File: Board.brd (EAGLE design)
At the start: 110.5 x 61 mm, 26 parts, among them IC1 BUF634U, IC2 LM555D, Q1 35A/25V/8.5mΩ, Q2 35A/25V/8.5mΩ, Q3 35A/25V/8.5mΩ, X3 MSTBV4

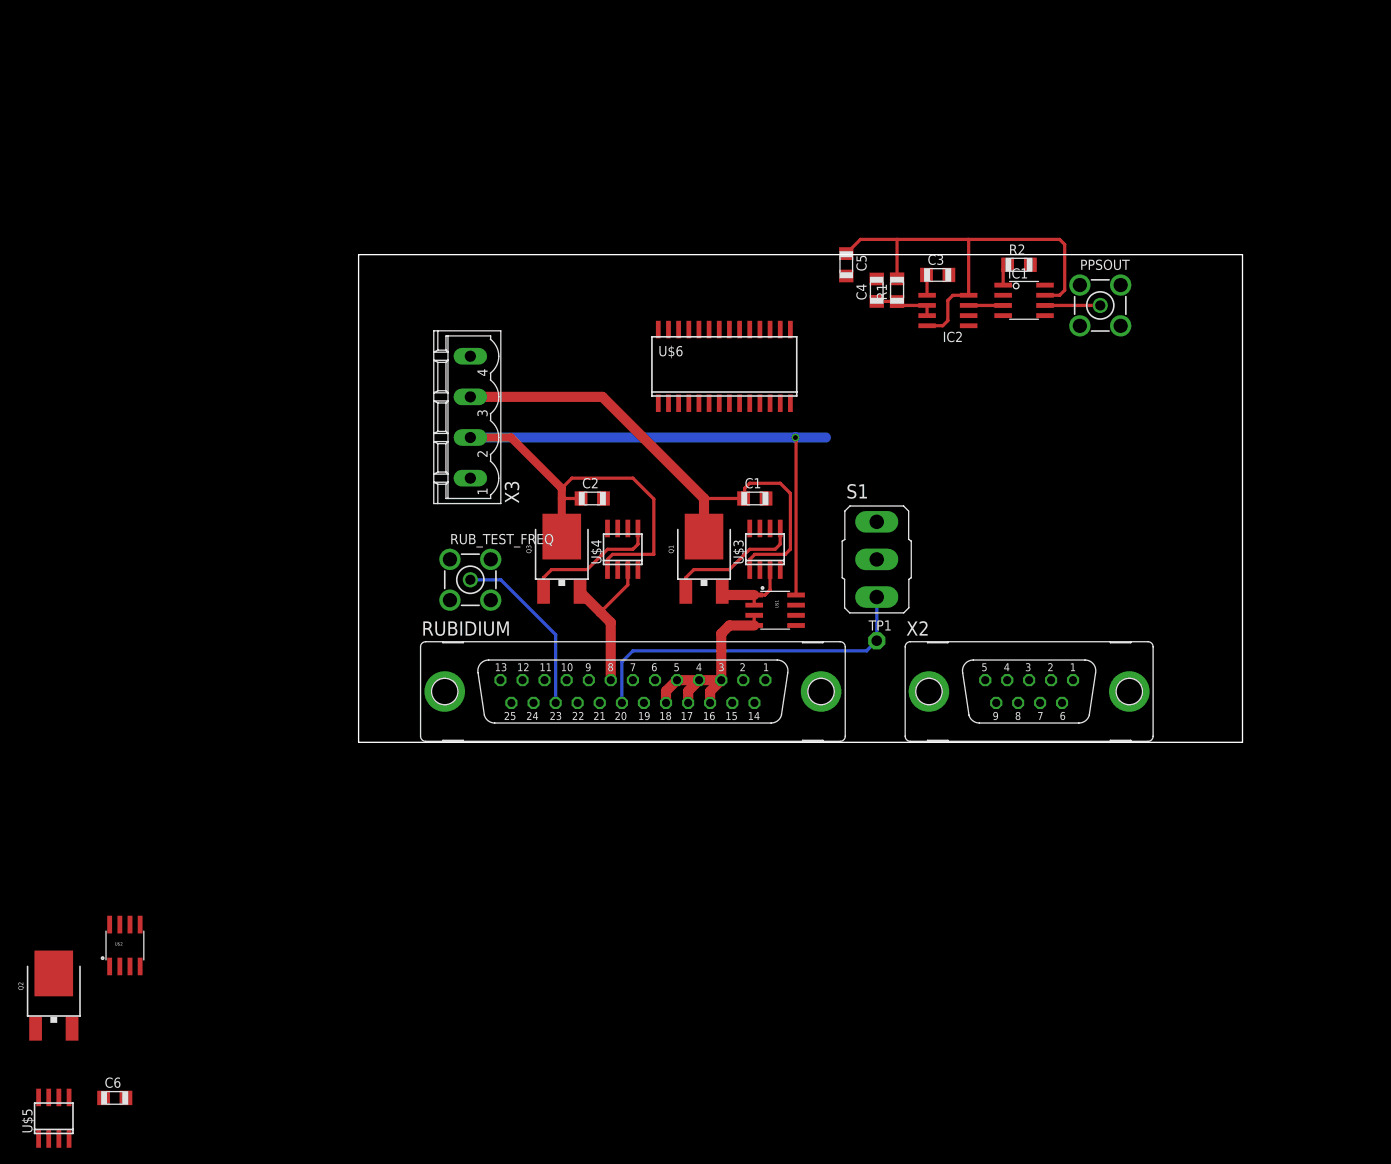
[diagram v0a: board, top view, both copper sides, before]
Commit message: PCB work
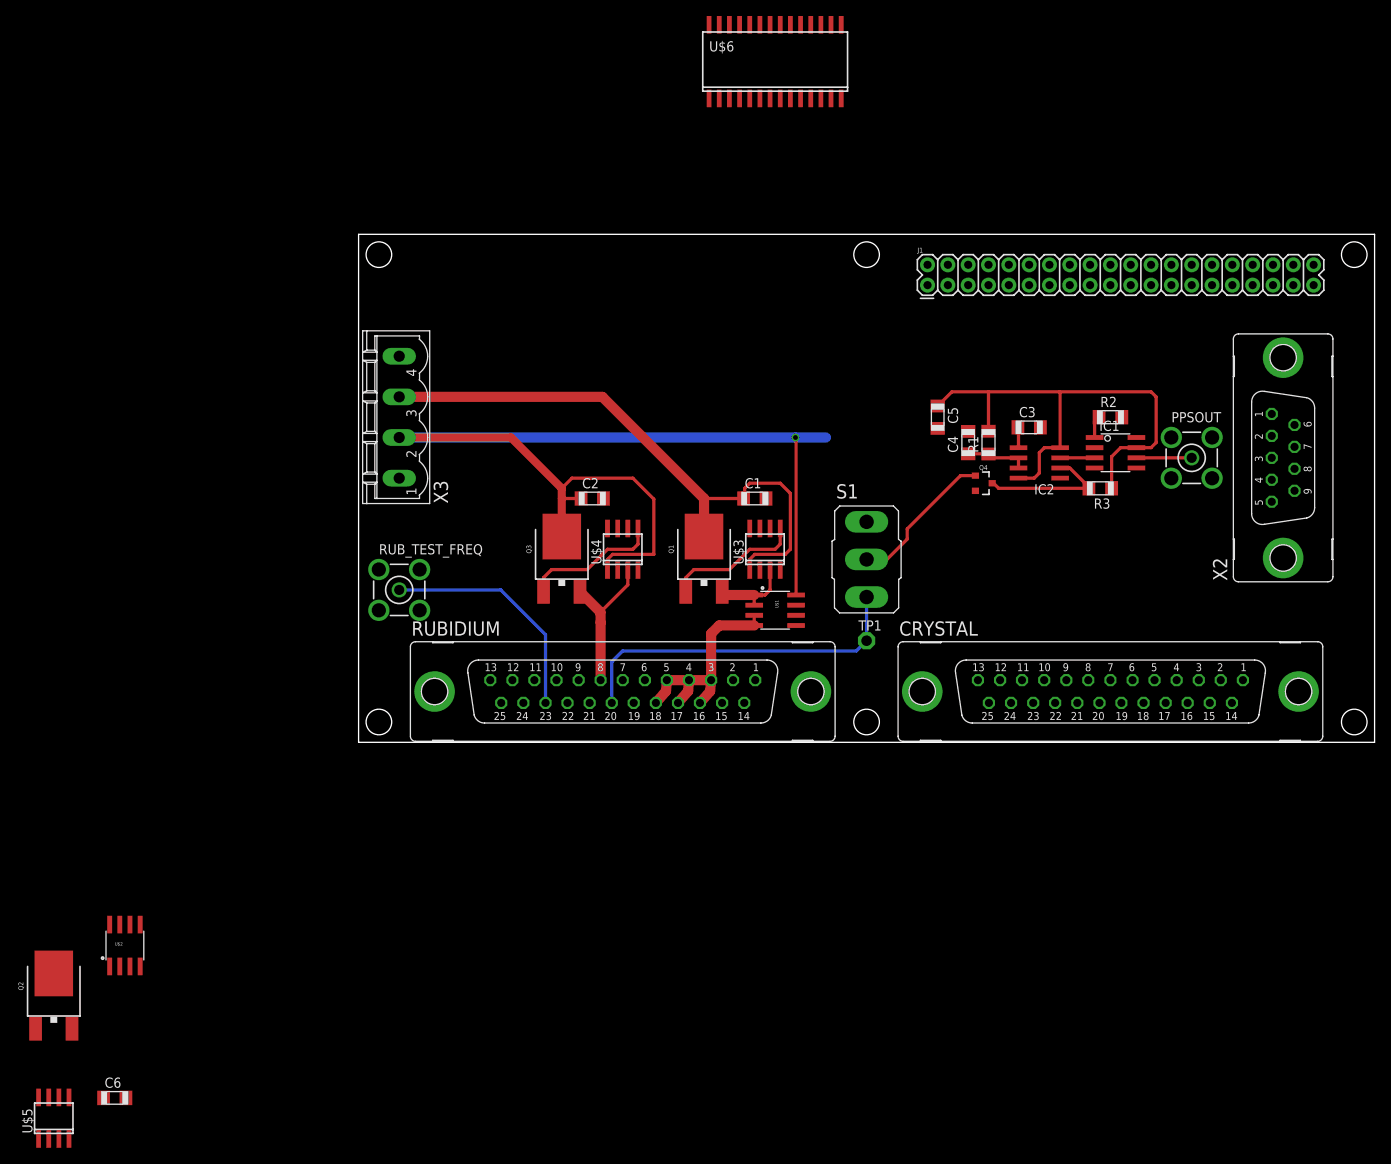
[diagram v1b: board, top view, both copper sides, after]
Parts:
- added CRYSTAL: (no value), con-subd:F25VP
- added J1: RASPBERRYPI-40-PIN-GPIO_PTH_NO_SHROUD, SparkFun-Connectors:2X20
- added Q4: 220mA/50V/3.5Ω, SparkFun-DiscreteSemi:SOT23-3
- added R3: 1k, resistor:R1206
- moved X2 43.1 mm to (115.6, 35.6), turned to 90 degrees
- moved U$6 38.6 mm to (52.1, 85.1)
- moved IC2 22.2 mm to (85.1, 34.9)
- moved C4 22.2 mm to (76.2, 37.5)
- moved PPSOUT 22.2 mm to (104.1, 35.6)
- moved R2 22.2 mm to (94.0, 40.6)
- moved C3 22.2 mm to (83.8, 39.4)
- moved C5 22.2 mm to (72.4, 40.6)
- moved IC1 22.2 mm to (94.6, 36.2)
- moved R1 22.2 mm to (78.7, 37.5)
- moved RUB_TEST_FREQ 8.98 mm to (5.08, 19.1)
- moved X3 8.89 mm to (5.08, 40.6)
- moved RUBIDIUM 1.27 mm to (33.0, 6.35)
- moved S1 1.27 mm to (63.5, 22.9)
- moved TP1 1.27 mm to (63.5, 12.7)
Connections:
- new net 3.3V: J1.1, J1.17
- new net 5V: J1.2, J1.4
- new net N$11: IC2.2, Q4.3, R3.2
- net +5V: now also R3.1
- net GND: now also J1.14, J1.20, J1.25, J1.30, J1.34, J1.39, J1.6, J1.9, Q4.2
- net RAWPPS: now also Q4.1
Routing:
- net +5V: track 171.0 -> 196.3 mm
- net RAWPPS: track 0.00 -> 18.7 mm
- net N$11: track 0.00 -> 17.1 mm
- net +15V: track 65.9 -> 74.8 mm
- net RUB_TEST_FREQ: track 22.0 -> 29.1 mm
- net RUBIDIUM_15: track 27.4 -> 28.4 mm
- net RUBIDIUM_5V: track 19.3 -> 18.8 mm
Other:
- board size 110.5 x 61 mm -> 127 x 63.5 mm
